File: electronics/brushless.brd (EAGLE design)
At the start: 36.8 x 56.2 mm, 66 parts, among them J1 USB_MINI-B_SMT, Q1 BUK7Y12-40E, Q2 BUK7Y12-40E, Q3 BUK7Y12-40E, Q4 BUK7Y12-40E, Q5 BUK7Y12-40E, Q6 BUK7Y12-40E, X1 JST-XH-10-PIN-LONG-PAD

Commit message: up
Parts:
- R23, R24, R25: value 15K -> 10K
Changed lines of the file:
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@@
 <element name="U$5" library="rhoban" package="CONNEC_1X08" value="CONNEC_1X08" x="18.415" y="1.905"/>
 <element name="X1" library="Rembrandt Electronics - JST XH Connectors v1-0" package="JST-XH-10-PACKAGE-LONG-PAD" value="JST-XH-10-PIN-LONG-PAD" x="17.145" y="44.45"/>
-<element name="R23" library="SparkFun-Resistors" package="0805" value="15K" x="31.75" y="27.94" rot="MR180">
+<element name="R23" library="SparkFun-Resistors" package="0805" value="10K" x="31.75" y="27.94" rot="MR180">
 <attribute name="PROD_ID" value=" " x="31.75" y="27.94" size="1.778" layer="28" rot="MR180" display="off"/>
 <attribute name="VALUE" value=" " x="31.75" y="27.94" size="1.778" layer="28" rot="MR180" display="off"/>
 </element>
-<element name="R24" library="SparkFun-Resistors" package="0805" value="15K" x="31.75" y="30.48" rot="MR180">
+<element name="R24" library="SparkFun-Resistors" package="0805" value="10K" x="31.75" y="30.48" rot="MR180">
 <attribute name="PROD_ID" value=" " x="31.75" y="30.48" size="1.778" layer="28" rot="MR180" display="off"/>
 <attribute name="VALUE" value=" " x="31.75" y="30.48" size="1.778" layer="28" rot="MR180" display="off"/>
 </element>
-<element name="R25" library="SparkFun-Resistors" package="0805" value="15K" x="31.75" y="33.02" rot="MR180">
+<element name="R25" library="SparkFun-Resistors" package="0805" value="10K" x="31.75" y="33.02" rot="MR180">
 <attribute name="PROD_ID" value=" " x="31.75" y="33.02" size="1.778" layer="28" rot="MR180" display="off"/>
 <attribute name="VALUE" value=" " x="31.75" y="33.02" size="1.778" layer="28" rot="MR180" display="off"/>

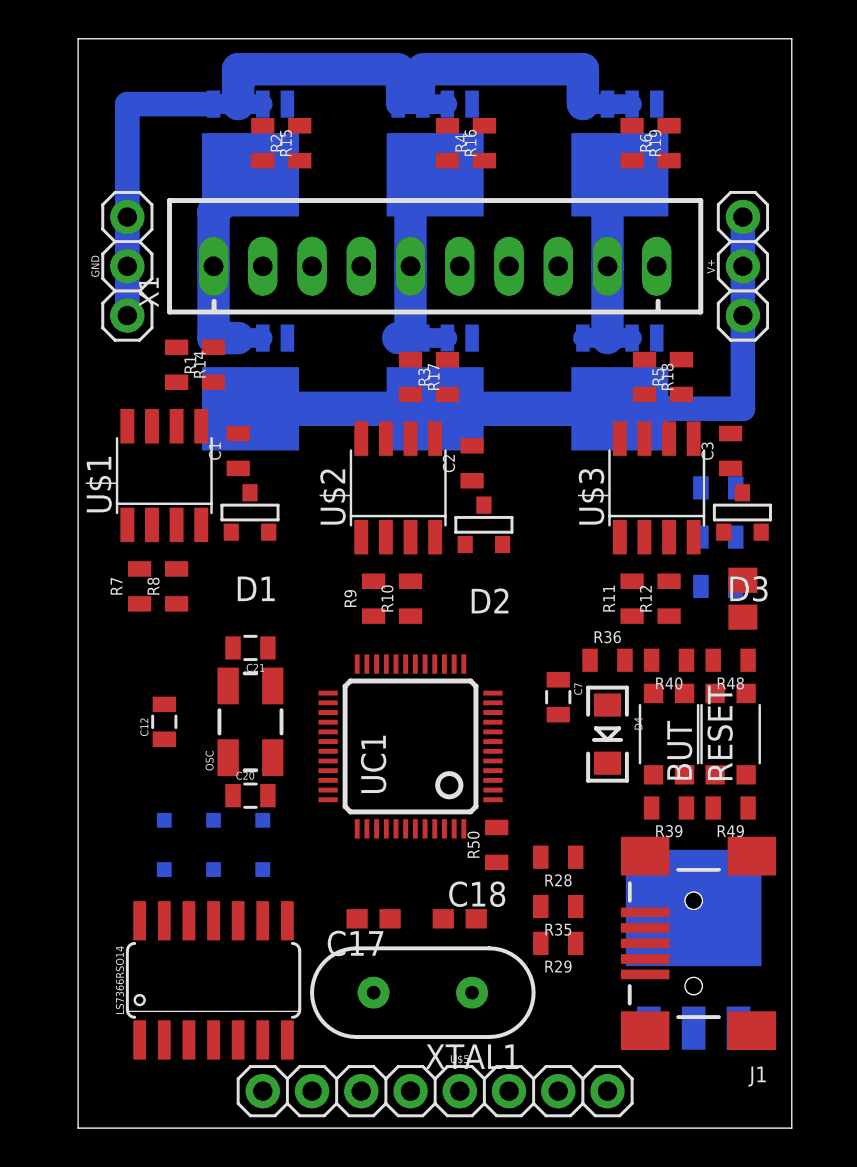
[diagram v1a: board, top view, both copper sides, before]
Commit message: wip
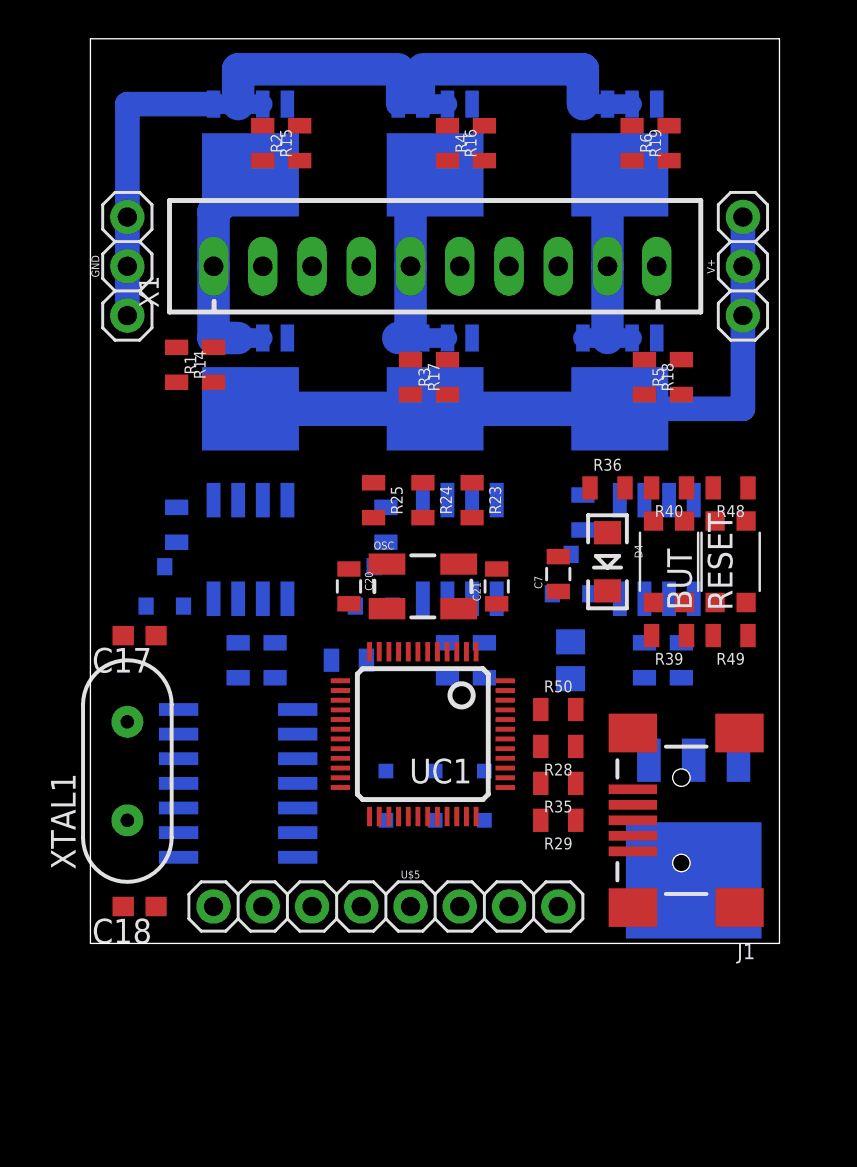
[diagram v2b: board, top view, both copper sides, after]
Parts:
- moved XTAL1 19.1 mm to (1.27, 18.4), turned to 90 degrees
- moved C17 18.9 mm to (1.91, 25.4)
- moved R25 17.8 mm to (14.0, 32.4), flipped to the top, turned to 270 degrees
- moved C18 16.5 mm to (1.91, 11.4), turned to 180 degrees
- moved R24 15.4 mm to (16.5, 32.4), flipped to the top, turned to 270 degrees
- moved R23 13.5 mm to (19.1, 32.4), flipped to the top, turned to 270 degrees
- moved C21 13.1 mm to (20.3, 27.9), turned to 90 degrees
- moved C20 11.9 mm to (12.7, 27.9), turned to 270 degrees
- moved PROGRAM 11.7 mm to (19.7, 18.4)
- moved OSC 11.3 mm to (16.5, 27.9), turned to 0 degrees
- moved ENC1 10.2 mm to (6.99, 17.8), flipped to the bottom, turned to 90 degrees
- moved C12 10.0 mm to (12.7, 24.1), flipped to the bottom, turned to 180 degrees
- moved U$5 9.86 mm to (15.9, 11.4)
- moved D3 9.44 mm to (24.1, 28.6), flipped to the bottom
- moved R13 9.44 mm to (24.1, 24.1), flipped to the bottom
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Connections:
- net RX1: now also UC1.31
- net TX1: now also UC1.30
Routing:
- net U_PHASE: track 11.7 -> 14.4 mm
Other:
- board size 36.8 x 56.2 mm -> 35.5 x 46.7 mm

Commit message: bl wip
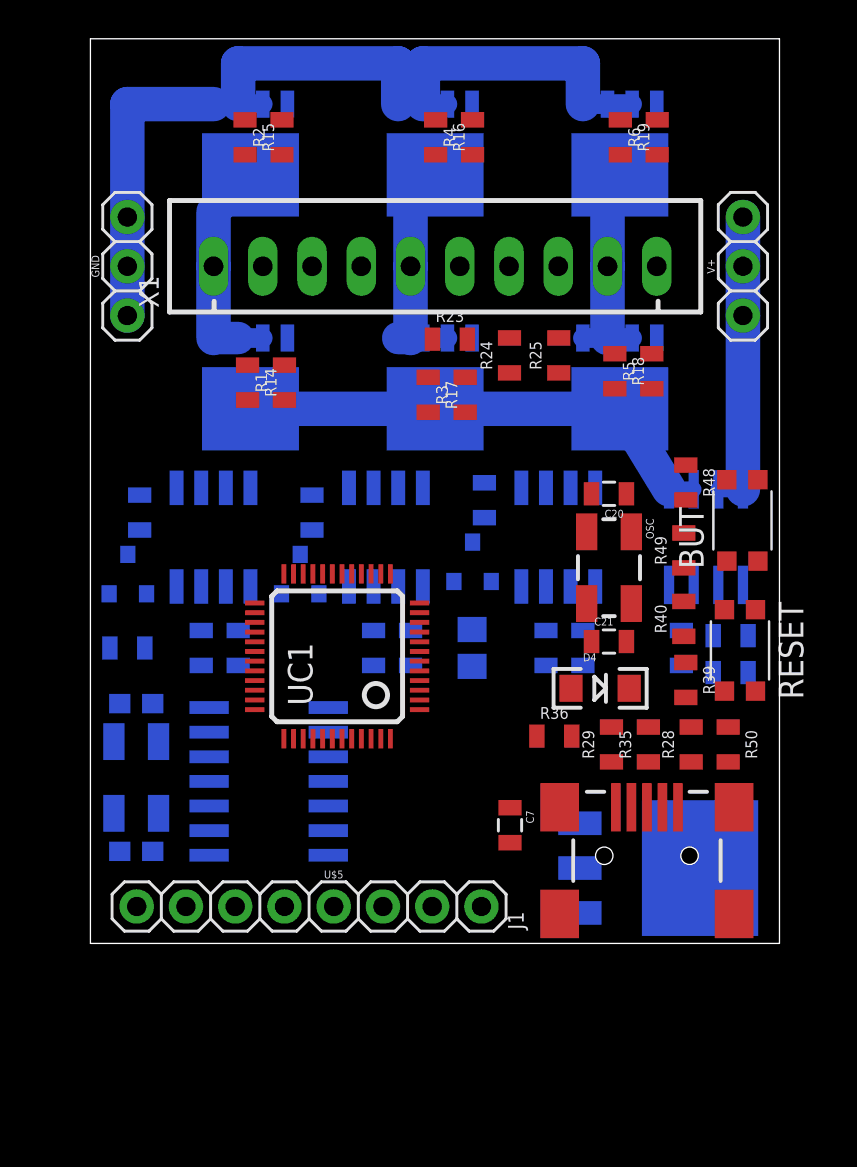
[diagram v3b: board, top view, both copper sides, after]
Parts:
- removed PROGRAM: CONNEC_1X066PADS, rhoban:6PADS
- removed XTAL1: 40Mhz, rhoban:HC49US
- added C4: 1nF, SparkFun-Passives:0805@1
- added OSC1: 40Mhz, SparkFun2:CRYSTAL-SMD-5X3
- added R20: 2K, SparkFun-Resistors:0805
- added R21: 3K, SparkFun-Resistors:0805
- added U$7: ACS712, rhoban:SO8
- moved C20 14.2 mm to (26.1, 32.7), turned to 180 degrees
- moved C7 13.2 mm to (21.0, 15.6), turned to 270 degrees
- moved R36 13.1 mm to (23.3, 20.2)
- moved R25 12.1 mm to (23.5, 39.9), turned to 90 degrees
- moved C12 11.4 mm to (1.27, 24.8)
- moved OSC 9.65 mm to (26.1, 28.9), turned to 270 degrees
- moved R50 8.95 mm to (32.3, 19.8), turned to 270 degrees
- moved R24 8.70 mm to (21.0, 39.9), turned to 90 degrees
- moved R23 8.38 mm to (17.9, 40.7), turned to 0 degrees
- moved R28 6.86 mm to (30.4, 19.8), turned to 90 degrees
- moved R40 6.80 mm to (30.0, 26.3), turned to 90 degrees
- moved D4 6.54 mm to (25.7, 22.7), turned to 0 degrees
- moved C21 6.45 mm to (26.1, 25.1), turned to 0 degrees
- moved UC1 5.97 mm to (12.1, 24.3), turned to 90 degrees
- moved RESET 5.86 mm to (32.9, 24.6)
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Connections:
- new net CUR: R20.2, R21.1, UC1.17
- new net N$24: R20.1, U$7.7
- new net N$27: C4.1, U$7.6
- new net V+_MOS: Q1.MB, Q3.MB, Q5.MB, U$7.1, U$7.2
- net 3.3: no longer PROGRAM.2
- net BOOT1: no longer PROGRAM.4
- net GND: now also C4.2, R21.2, U$7.5; no longer PROGRAM.1
- net N$20: now also OSC1.1; no longer XTAL1.2
- net N$21: now also OSC1.3; no longer XTAL1.1
- net RESET: no longer PROGRAM.3
- net RX1: no longer PROGRAM.6
- net TX1: no longer PROGRAM.5
- net V+: now also U$7.3, U$7.4; no longer Q1.MB, Q3.MB, Q5.MB
- net VCC: now also U$7.8
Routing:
- net V+_MOS: track 0.00 -> 25.2 mm
- net V+: track 35.3 -> 15.3 mm
- net GND: track 46.7 -> 47.9 mm
